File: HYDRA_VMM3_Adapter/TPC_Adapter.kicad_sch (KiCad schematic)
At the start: 1 part

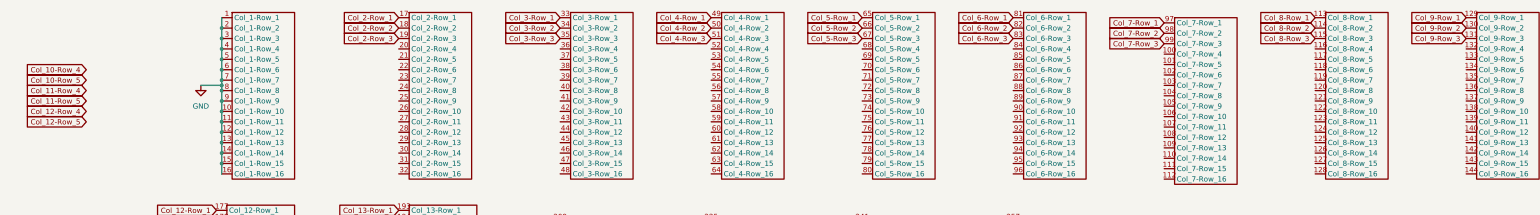
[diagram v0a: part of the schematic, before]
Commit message: .
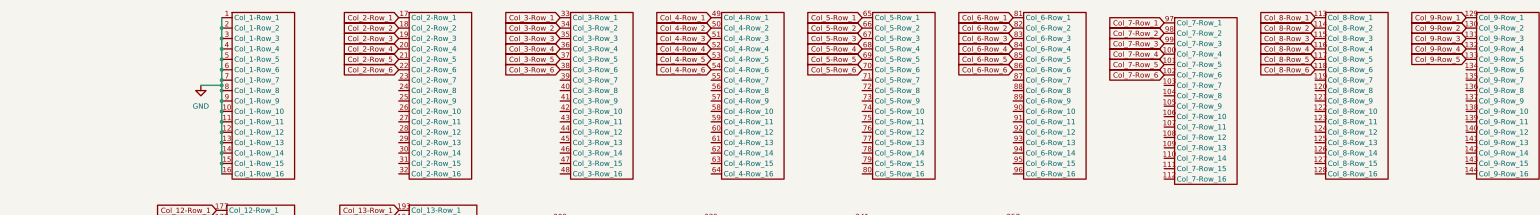
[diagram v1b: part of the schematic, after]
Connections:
- net Col_7-Row_4: now reaches U1.100 (Col_7-Row_4)
- net Col_7-Row_5: now reaches U1.101 (Col_7-Row_5)
- net Col_7-Row_6: now reaches U1.102 (Col_7-Row_6)
- net Col_8-Row_4: now reaches U1.116 (Col_8-Row_4)
- net Col_8-Row_5: now reaches U1.117 (Col_8-Row_5)
- net Col_8-Row_6: now reaches U1.118 (Col_8-Row_6)
- net Col_9-Row_4: now reaches U1.132 (Col_9-Row_4)
- net Col_9-Row_5: now reaches U1.133 (Col_9-Row_5)
- net Col_2-Row_4: now reaches U1.20 (Col_2-Row_4)
- net Col_2-Row_5: now reaches U1.21 (Col_2-Row_5)
- net Col_2-Row_6: now reaches U1.22 (Col_2-Row_6)
- net Col_3-Row_4: now reaches U1.36 (Col_3-Row_4)
- net Col_3-Row_5: now reaches U1.37 (Col_3-Row_5)
- net Col_3-Row_6: now reaches U1.38 (Col_3-Row_6)
- net Col_4-Row_4: now reaches U1.52 (Col_4-Row_4)
- net Col_4-Row_5: now reaches U1.53 (Col_4-Row_5)
- net Col_4-Row_6: now reaches U1.54 (Col_4-Row_6)
- net Col_5-Row_4: now reaches U1.68 (Col_5-Row_4)
- net Col_5-Row_5: now reaches U1.69 (Col_5-Row_5)
- net Col_5-Row_6: now reaches U1.70 (Col_5-Row_6)
- net Col_6-Row_4: now reaches U1.84 (Col_6-Row_4)
- net Col_6-Row_5: now reaches U1.85 (Col_6-Row_5)
- net Col_6-Row_6: now reaches U1.86 (Col_6-Row_6)

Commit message: .
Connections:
- net Col_23-Row_1: now reaches U1.353 (Col_23-Row_1)
- net Col_23-Row_2: now reaches U1.354 (Col_23-Row_2)
- net Col_23-Row_3: now reaches U1.355 (Col_23-Row_3)
- net Col_23-Row_4: now reaches U1.356 (Col_23-Row_4)
- net Col_23-Row_5: now reaches U1.357 (Col_23-Row_5)
- net Col_24-Row_1: now reaches U1.369 (Col_24-Row_1)
- net Col_24-Row_2: now reaches U1.370 (Col_24-Row_2)
- net Col_24-Row_3: now reaches U1.371 (Col_24-Row_3)
- net Col_24-Row_4: now reaches U1.372 (Col_24-Row_4)
- net Col_24-Row_5: now reaches U1.373 (Col_24-Row_5)
- net Col_25-Row_1: now reaches U1.385 (Col_25-Row_1)
- net Col_25-Row_2: now reaches U1.386 (Col_25-Row_2)
- net Col_25-Row_3: now reaches U1.387 (Col_25-Row_3)
- net Col_25-Row_4: now reaches U1.388 (Col_25-Row_4)
- net Col_25-Row_5: now reaches U1.389 (Col_25-Row_5)
- net Col_26-Row_1: now reaches U1.401 (Col_26-Row_1)
- net Col_26-Row_2: now reaches U1.402 (Col_26-Row_2)
- net Col_26-Row_3: now reaches U1.403 (Col_26-Row_3)
- net Col_26-Row_4: now reaches U1.404 (Col_26-Row_4)
- net Col_26-Row_5: now reaches U1.405 (Col_26-Row_5)
- net Col_27-Row_1: now reaches U1.417 (Col_27-Row_1)
- net Col_27-Row_2: now reaches U1.418 (Col_27-Row_2)
- net Col_27-Row_3: now reaches U1.419 (Col_27-Row_3)
- net Col_27-Row_4: now reaches U1.420 (Col_27-Row_4)
- net Col_27-Row_5: now reaches U1.421 (Col_27-Row_5)
- net Col_28-Row_1: now reaches U1.433 (Col_28-Row_1)
- net Col_28-Row_2: now reaches U1.434 (Col_28-Row_2)
- net Col_28-Row_3: now reaches U1.435 (Col_28-Row_3)
- net Col_28-Row_4: now reaches U1.436 (Col_28-Row_4)
- net Col_28-Row_5: now reaches U1.437 (Col_28-Row_5)
- net Col_29-Row_1: now reaches U1.449 (Col_29-Row_1)
- net Col_29-Row_2: now reaches U1.450 (Col_29-Row_2)
- net Col_29-Row_3: now reaches U1.451 (Col_29-Row_3)
- net Col_29-Row_4: now reaches U1.452 (Col_29-Row_4)
- net Col_29-Row_5: now reaches U1.453 (Col_29-Row_5)
- net Col_30-Row_1: now reaches U1.465 (Col_30-Row_1)
- net Col_30-Row_2: now reaches U1.466 (Col_30-Row_2)
- net Col_30-Row_3: now reaches U1.467 (Col_30-Row_3)
- net Col_30-Row_4: now reaches U1.468 (Col_30-Row_4)
- net Col_30-Row_5: now reaches U1.469 (Col_30-Row_5)
- net Col_31-Row_1: now reaches U1.481 (Col_31-Row_1)
- net Col_31-Row_2: now reaches U1.482 (Col_31-Row_2)
- net Col_31-Row_3: now reaches U1.483 (Col_31-Row_3)
- net Col_31-Row_4: now reaches U1.484 (Col_31-Row_4)
- net Col_31-Row_5: now reaches U1.485 (Col_31-Row_5)
- net Col_32-Row_1: now reaches U1.497 (Col_32-Row_1)
- net Col_32-Row_2: now reaches U1.498 (Col_32-Row_2)
- net Col_32-Row_3: now reaches U1.499 (Col_32-Row_3)
- net Col_32-Row_4: now reaches U1.500 (Col_32-Row_4)
- net Col_32-Row_5: now reaches U1.501 (Col_32-Row_5)
- net Col_33-Row_1: now reaches U1.513 (Col_33-Row_1)
- net Col_33-Row_2: now reaches U1.514 (Col_33-Row_2)
- net Col_33-Row_3: now reaches U1.515 (Col_33-Row_3)
- net Col_33-Row_4: now reaches U1.516 (Col_33-Row_4)
- net Col_33-Row_5: now reaches U1.517 (Col_33-Row_5)
- net Col_34-Row_1: now reaches U1.529 (Col_34-Row_1)
- net Col_34-Row_2: now reaches U1.530 (Col_34-Row_2)
- net Col_34-Row_3: now reaches U1.531 (Col_34-Row_3)
- net Col_34-Row_4: now reaches U1.532 (Col_34-Row_4)
- net Col_34-Row_5: now reaches U1.533 (Col_34-Row_5)
- net Col_35-Row_1: now reaches U1.545 (Col_35-Row_1)
- net Col_35-Row_2: now reaches U1.546 (Col_35-Row_2)
- net Col_35-Row_3: now reaches U1.547 (Col_35-Row_3)
- net Col_35-Row_4: now reaches U1.548 (Col_35-Row_4)
- net Col_35-Row_5: now reaches U1.549 (Col_35-Row_5)
- net Col_36-Row_1: now reaches U1.561 (Col_36-Row_1)
- net Col_36-Row_2: now reaches U1.562 (Col_36-Row_2)
- net Col_36-Row_3: now reaches U1.563 (Col_36-Row_3)
- net Col_36-Row_4: now reaches U1.564 (Col_36-Row_4)
- net Col_36-Row_5: now reaches U1.565 (Col_36-Row_5)
- net Col_37-Row_1: now reaches U1.577 (Col_37-Row_1)
- net Col_37-Row_2: now reaches U1.578 (Col_37-Row_2)
- net Col_37-Row_3: now reaches U1.579 (Col_37-Row_3)
- net Col_37-Row_4: now reaches U1.580 (Col_37-Row_4)
- net Col_37-Row_5: now reaches U1.581 (Col_37-Row_5)
- net Col_37-Row_6: now reaches U1.582 (Col_37-Row_6)
- net Col_38-Row_1: now reaches U1.593 (Col_38-Row_1)
- net Col_38-Row_2: now reaches U1.594 (Col_38-Row_2)
- net Col_38-Row_3: now reaches U1.595 (Col_38-Row_3)
- net Col_38-Row_4: now reaches U1.596 (Col_38-Row_4)
- net Col_38-Row_5: now reaches U1.597 (Col_38-Row_5)
- net Col_38-Row_6: now reaches U1.598 (Col_38-Row_6)
- net Col_39-Row_1: now reaches U1.609 (Col_39-Row_1)
- net Col_39-Row_2: now reaches U1.610 (Col_39-Row_2)
- net Col_39-Row_3: now reaches U1.611 (Col_39-Row_3)
- net Col_39-Row_4: now reaches U1.612 (Col_39-Row_4)
- net Col_39-Row_5: now reaches U1.613 (Col_39-Row_5)
- net Col_39-Row_6: now reaches U1.614 (Col_39-Row_6)
- net Col_40-Row_1: now reaches U1.625 (Col_40-Row_1)
- net Col_40-Row_2: now reaches U1.626 (Col_40-Row_2)
- net Col_40-Row_3: now reaches U1.627 (Col_40-Row_3)
- net Col_40-Row_4: now reaches U1.628 (Col_40-Row_4)
- net Col_40-Row_5: now reaches U1.629 (Col_40-Row_5)
- net Col_40-Row_6: now reaches U1.630 (Col_40-Row_6)
- net Col_41-Row_1: now reaches U1.641 (Col_41-Row_1)
- net Col_41-Row_2: now reaches U1.642 (Col_41-Row_2)
- net Col_41-Row_3: now reaches U1.643 (Col_41-Row_3)
- net Col_41-Row_4: now reaches U1.644 (Col_41-Row_4)
- net Col_41-Row_5: now reaches U1.645 (Col_41-Row_5)
- net Col_41-Row_6: now reaches U1.646 (Col_41-Row_6)
- net Col_42-Row_1: now reaches U1.657 (Col_42-Row_1)
- net Col_42-Row_2: now reaches U1.658 (Col_42-Row_2)
- net Col_42-Row_3: now reaches U1.659 (Col_42-Row_3)
- net Col_42-Row_4: now reaches U1.660 (Col_42-Row_4)
- net Col_42-Row_5: now reaches U1.661 (Col_42-Row_5)
- net Col_42-Row_6: now reaches U1.662 (Col_42-Row_6)
- net Col_43-Row_1: now reaches U1.673 (Col_43-Row_1)
- net Col_43-Row_2: now reaches U1.674 (Col_43-Row_2)
- net Col_43-Row_3: now reaches U1.675 (Col_43-Row_3)
- net Col_43-Row_4: now reaches U1.676 (Col_43-Row_4)
- net Col_43-Row_5: now reaches U1.677 (Col_43-Row_5)
- net Col_43-Row_6: now reaches U1.678 (Col_43-Row_6)

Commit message: .
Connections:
- net Col_7-Row_12: now reaches U1.108 (Col_7-Row_12)
- net Col_7-Row_13: now reaches U1.109 (Col_7-Row_13)
- net Col_7-Row_14: now reaches U1.110 (Col_7-Row_14)
- net Col_7-Row_15: now reaches U1.111 (Col_7-Row_15)
- net Col_7-Row_16: now reaches U1.112 (Col_7-Row_16)
- net Col_8-Row_12: now reaches U1.124 (Col_8-Row_12)
- net Col_8-Row_13: now reaches U1.125 (Col_8-Row_13)
- net Col_8-Row_14: now reaches U1.126 (Col_8-Row_14)
- net Col_8-Row_15: now reaches U1.127 (Col_8-Row_15)
- net Col_8-Row_16: now reaches U1.128 (Col_8-Row_16)
- net Col_9-Row_12: now reaches U1.140 (Col_9-Row_12)
- net Col_9-Row_13: now reaches U1.141 (Col_9-Row_13)
- net Col_9-Row_14: now reaches U1.142 (Col_9-Row_14)
- net Col_9-Row_15: now reaches U1.143 (Col_9-Row_15)
- net Col_9-Row_16: now reaches U1.144 (Col_9-Row_16)
- net Col_10-Row_12: now reaches U1.156 (Col_10-Row_12)
- net Col_10-Row_13: now reaches U1.157 (Col_10-Row_13)
- net Col_10-Row_14: now reaches U1.158 (Col_10-Row_14)
- net Col_10-Row_15: now reaches U1.159 (Col_10-Row_15)
- net Col_10-Row_16: now reaches U1.160 (Col_10-Row_16)
- net Col_11-Row_12: now reaches U1.172 (Col_11-Row_12)
- net Col_11-Row_13: now reaches U1.173 (Col_11-Row_13)
- net Col_11-Row_14: now reaches U1.174 (Col_11-Row_14)
- net Col_11-Row_15: now reaches U1.175 (Col_11-Row_15)
- net Col_11-Row_16: now reaches U1.176 (Col_11-Row_16)
- net Col_12-Row_12: now reaches U1.188 (Col_12-Row_12)
- net Col_12-Row_13: now reaches U1.189 (Col_12-Row_13)
- net Col_12-Row_14: now reaches U1.190 (Col_12-Row_14)
- net Col_12-Row_15: now reaches U1.191 (Col_12-Row_15)
- net Col_12-Row_16: now reaches U1.192 (Col_12-Row_16)
- net Col_13-Row_12: now reaches U1.204 (Col_13-Row_12)
- net Col_13-Row_13: now reaches U1.205 (Col_13-Row_13)
- net Col_13-Row_14: now reaches U1.206 (Col_13-Row_14)
- net Col_13-Row_15: now reaches U1.207 (Col_13-Row_15)
- net Col_13-Row_16: now reaches U1.208 (Col_13-Row_16)
- net Col_14-Row_12: now reaches U1.220 (Col_14-Row_12)
- net Col_14-Row_13: now reaches U1.221 (Col_14-Row_13)
- net Col_14-Row_14: now reaches U1.222 (Col_14-Row_14)
- net Col_14-Row_15: now reaches U1.223 (Col_14-Row_15)
- net Col_14-Row_16: now reaches U1.224 (Col_14-Row_16)
- net Col_15-Row_12: now reaches U1.236 (Col_15-Row_12)
- net Col_15-Row_13: now reaches U1.237 (Col_15-Row_13)
- net Col_15-Row_14: now reaches U1.238 (Col_15-Row_14)
- net Col_15-Row_15: now reaches U1.239 (Col_15-Row_15)
- net Col_15-Row_16: now reaches U1.240 (Col_15-Row_16)
- net Col_16-Row_11: now reaches U1.251 (Col_16-Row_11)
- net Col_16-Row_12: now reaches U1.252 (Col_16-Row_12)
- net Col_16-Row_13: now reaches U1.253 (Col_16-Row_13)
- net Col_16-Row_14: now reaches U1.254 (Col_16-Row_14)
- net Col_16-Row_15: now reaches U1.255 (Col_16-Row_15)
- net Col_16-Row_16: now reaches U1.256 (Col_16-Row_16)
- net Col_17-Row_11: now reaches U1.267 (Col_17-Row_11)
- net Col_17-Row_12: now reaches U1.268 (Col_17-Row_12)
- net Col_17-Row_13: now reaches U1.269 (Col_17-Row_13)
- net Col_17-Row_14: now reaches U1.270 (Col_17-Row_14)
- net Col_17-Row_15: now reaches U1.271 (Col_17-Row_15)
- net Col_17-Row_16: now reaches U1.272 (Col_17-Row_16)
- net Col_2-Row_12: now reaches U1.28 (Col_2-Row_12)
- net Col_18-Row_11: now reaches U1.283 (Col_18-Row_11)
- net Col_18-Row_12: now reaches U1.284 (Col_18-Row_12)
- net Col_18-Row_13: now reaches U1.285 (Col_18-Row_13)
- net Col_18-Row_14: now reaches U1.286 (Col_18-Row_14)
- net Col_18-Row_15: now reaches U1.287 (Col_18-Row_15)
- net Col_18-Row_16: now reaches U1.288 (Col_18-Row_16)
- net Col_2-Row_13: now reaches U1.29 (Col_2-Row_13)
- net Col_19-Row_11: now reaches U1.299 (Col_19-Row_11)
- net Col_2-Row_14: now reaches U1.30 (Col_2-Row_14)
- net Col_19-Row_12: now reaches U1.300 (Col_19-Row_12)
- net Col_19-Row_13: now reaches U1.301 (Col_19-Row_13)
- net Col_19-Row_14: now reaches U1.302 (Col_19-Row_14)
- net Col_19-Row_15: now reaches U1.303 (Col_19-Row_15)
- net Col_19-Row_16: now reaches U1.304 (Col_19-Row_16)
- net Col_2-Row_15: now reaches U1.31 (Col_2-Row_15)
- net Col_20-Row_11: now reaches U1.315 (Col_20-Row_11)
- net Col_20-Row_12: now reaches U1.316 (Col_20-Row_12)
- net Col_20-Row_13: now reaches U1.317 (Col_20-Row_13)
- net Col_20-Row_14: now reaches U1.318 (Col_20-Row_14)
- net Col_20-Row_15: now reaches U1.319 (Col_20-Row_15)
- net Col_2-Row_16: now reaches U1.32 (Col_2-Row_16)
- net Col_20-Row_16: now reaches U1.320 (Col_20-Row_16)
- net Col_21-Row_11: now reaches U1.331 (Col_21-Row_11)
- net Col_21-Row_12: now reaches U1.332 (Col_21-Row_12)
- net Col_21-Row_13: now reaches U1.333 (Col_21-Row_13)
- net Col_21-Row_14: now reaches U1.334 (Col_21-Row_14)
- net Col_21-Row_15: now reaches U1.335 (Col_21-Row_15)
- net Col_21-Row_16: now reaches U1.336 (Col_21-Row_16)
- net Col_22-Row_11: now reaches U1.347 (Col_22-Row_11)
- net Col_22-Row_12: now reaches U1.348 (Col_22-Row_12)
- net Col_22-Row_13: now reaches U1.349 (Col_22-Row_13)
- net Col_22-Row_14: now reaches U1.350 (Col_22-Row_14)
- net Col_22-Row_15: now reaches U1.351 (Col_22-Row_15)
- net Col_22-Row_16: now reaches U1.352 (Col_22-Row_16)
- net Col_3-Row_12: now reaches U1.44 (Col_3-Row_12)
- net Col_3-Row_13: now reaches U1.45 (Col_3-Row_13)
- net Col_3-Row_14: now reaches U1.46 (Col_3-Row_14)
- net Col_3-Row_15: now reaches U1.47 (Col_3-Row_15)
- net Col_3-Row_16: now reaches U1.48 (Col_3-Row_16)
- net Col_4-Row_12: now reaches U1.60 (Col_4-Row_12)
- net Col_4-Row_13: now reaches U1.61 (Col_4-Row_13)
- net Col_4-Row_14: now reaches U1.62 (Col_4-Row_14)
- net Col_4-Row_15: now reaches U1.63 (Col_4-Row_15)
- net Col_4-Row_16: now reaches U1.64 (Col_4-Row_16)
- net Col_5-Row_12: now reaches U1.76 (Col_5-Row_12)
- net Col_5-Row_13: now reaches U1.77 (Col_5-Row_13)
- net Col_5-Row_14: now reaches U1.78 (Col_5-Row_14)
- net Col_5-Row_15: now reaches U1.79 (Col_5-Row_15)
- net Col_5-Row_16: now reaches U1.80 (Col_5-Row_16)
- net Col_6-Row_12: now reaches U1.92 (Col_6-Row_12)
- net Col_6-Row_13: now reaches U1.93 (Col_6-Row_13)
- net Col_6-Row_14: now reaches U1.94 (Col_6-Row_14)
- net Col_6-Row_15: now reaches U1.95 (Col_6-Row_15)
- net Col_6-Row_16: now reaches U1.96 (Col_6-Row_16)

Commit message: .
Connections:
- net Col_23-Row_11: now reaches U1.363 (Col_23-Row_11)
- net Col_23-Row_12: now reaches U1.364 (Col_23-Row_12)
- net Col_23-Row_13: now reaches U1.365 (Col_23-Row_13)
- net Col_23-Row_14: now reaches U1.366 (Col_23-Row_14)
- net Col_23-Row_15: now reaches U1.367 (Col_23-Row_15)
- net Col_23-Row_16: now reaches U1.368 (Col_23-Row_16)
- net Col_24-Row_11: now reaches U1.379 (Col_24-Row_11)
- net Col_24-Row_12: now reaches U1.380 (Col_24-Row_12)
- net Col_24-Row_13: now reaches U1.381 (Col_24-Row_13)
- net Col_24-Row_14: now reaches U1.382 (Col_24-Row_14)
- net Col_24-Row_15: now reaches U1.383 (Col_24-Row_15)
- net Col_24-Row_16: now reaches U1.384 (Col_24-Row_16)
- net Col_25-Row_11: now reaches U1.395 (Col_25-Row_11)
- net Col_25-Row_12: now reaches U1.396 (Col_25-Row_12)
- net Col_25-Row_13: now reaches U1.397 (Col_25-Row_13)
- net Col_25-Row_14: now reaches U1.398 (Col_25-Row_14)
- net Col_25-Row_15: now reaches U1.399 (Col_25-Row_15)
- net Col_25-Row_16: now reaches U1.400 (Col_25-Row_16)
- net Col_26-Row_11: now reaches U1.411 (Col_26-Row_11)
- net Col_26-Row_12: now reaches U1.412 (Col_26-Row_12)
- net Col_26-Row_13: now reaches U1.413 (Col_26-Row_13)
- net Col_26-Row_14: now reaches U1.414 (Col_26-Row_14)
- net Col_26-Row_15: now reaches U1.415 (Col_26-Row_15)
- net Col_26-Row_16: now reaches U1.416 (Col_26-Row_16)
- net Col_27-Row_11: now reaches U1.427 (Col_27-Row_11)
- net Col_27-Row_12: now reaches U1.428 (Col_27-Row_12)
- net Col_27-Row_13: now reaches U1.429 (Col_27-Row_13)
- net Col_27-Row_14: now reaches U1.430 (Col_27-Row_14)
- net Col_27-Row_15: now reaches U1.431 (Col_27-Row_15)
- net Col_27-Row_16: now reaches U1.432 (Col_27-Row_16)
- net Col_28-Row_11: now reaches U1.443 (Col_28-Row_11)
- net Col_28-Row_12: now reaches U1.444 (Col_28-Row_12)
- net Col_28-Row_13: now reaches U1.445 (Col_28-Row_13)
- net Col_28-Row_14: now reaches U1.446 (Col_28-Row_14)
- net Col_28-Row_15: now reaches U1.447 (Col_28-Row_15)
- net Col_28-Row_16: now reaches U1.448 (Col_28-Row_16)
- net Col_29-Row_11: now reaches U1.459 (Col_29-Row_11)
- net Col_29-Row_12: now reaches U1.460 (Col_29-Row_12)
- net Col_29-Row_13: now reaches U1.461 (Col_29-Row_13)
- net Col_29-Row_14: now reaches U1.462 (Col_29-Row_14)
- net Col_29-Row_15: now reaches U1.463 (Col_29-Row_15)
- net Col_29-Row_16: now reaches U1.464 (Col_29-Row_16)
- net Col_30-Row_12: now reaches U1.476 (Col_30-Row_12)
- net Col_30-Row_13: now reaches U1.477 (Col_30-Row_13)
- net Col_30-Row_14: now reaches U1.478 (Col_30-Row_14)
- net Col_30-Row_15: now reaches U1.479 (Col_30-Row_15)
- net Col_30-Row_16: now reaches U1.480 (Col_30-Row_16)
- net Col_31-Row_12: now reaches U1.492 (Col_31-Row_12)
- net Col_31-Row_13: now reaches U1.493 (Col_31-Row_13)
- net Col_31-Row_14: now reaches U1.494 (Col_31-Row_14)
- net Col_31-Row_15: now reaches U1.495 (Col_31-Row_15)
- net Col_31-Row_16: now reaches U1.496 (Col_31-Row_16)
- net Col_32-Row_12: now reaches U1.508 (Col_32-Row_12)
- net Col_32-Row_13: now reaches U1.509 (Col_32-Row_13)
- net Col_32-Row_14: now reaches U1.510 (Col_32-Row_14)
- net Col_32-Row_15: now reaches U1.511 (Col_32-Row_15)
- net Col_32-Row_16: now reaches U1.512 (Col_32-Row_16)
- net Col_33-Row_12: now reaches U1.524 (Col_33-Row_12)
- net Col_33-Row_13: now reaches U1.525 (Col_33-Row_13)
- net Col_33-Row_14: now reaches U1.526 (Col_33-Row_14)
- net Col_33-Row_15: now reaches U1.527 (Col_33-Row_15)
- net Col_33-Row_16: now reaches U1.528 (Col_33-Row_16)
- net Col_34-Row_12: now reaches U1.540 (Col_34-Row_12)
- net Col_34-Row_13: now reaches U1.541 (Col_34-Row_13)
- net Col_34-Row_14: now reaches U1.542 (Col_34-Row_14)
- net Col_34-Row_15: now reaches U1.543 (Col_34-Row_15)
- net Col_34-Row_16: now reaches U1.544 (Col_34-Row_16)
- net Col_35-Row_12: now reaches U1.556 (Col_35-Row_12)
- net Col_35-Row_13: now reaches U1.557 (Col_35-Row_13)
- net Col_35-Row_14: now reaches U1.558 (Col_35-Row_14)
- net Col_35-Row_15: now reaches U1.559 (Col_35-Row_15)
- net Col_35-Row_16: now reaches U1.560 (Col_35-Row_16)
- net Col_36-Row_12: now reaches U1.572 (Col_36-Row_12)
- net Col_36-Row_13: now reaches U1.573 (Col_36-Row_13)
- net Col_36-Row_14: now reaches U1.574 (Col_36-Row_14)
- net Col_36-Row_15: now reaches U1.575 (Col_36-Row_15)
- net Col_36-Row_16: now reaches U1.576 (Col_36-Row_16)
- net Col_37-Row_12: now reaches U1.588 (Col_37-Row_12)
- net Col_37-Row_13: now reaches U1.589 (Col_37-Row_13)
- net Col_37-Row_14: now reaches U1.590 (Col_37-Row_14)
- net Col_37-Row_15: now reaches U1.591 (Col_37-Row_15)
- net Col_37-Row_16: now reaches U1.592 (Col_37-Row_16)
- net Col_38-Row_12: now reaches U1.604 (Col_38-Row_12)
- net Col_38-Row_13: now reaches U1.605 (Col_38-Row_13)
- net Col_38-Row_14: now reaches U1.606 (Col_38-Row_14)
- net Col_38-Row_15: now reaches U1.607 (Col_38-Row_15)
- net Col_38-Row_16: now reaches U1.608 (Col_38-Row_16)
- net Col_39-Row_12: now reaches U1.620 (Col_39-Row_12)
- net Col_39-Row_13: now reaches U1.621 (Col_39-Row_13)
- net Col_39-Row_14: now reaches U1.622 (Col_39-Row_14)
- net Col_39-Row_15: now reaches U1.623 (Col_39-Row_15)
- net Col_39-Row_16: now reaches U1.624 (Col_39-Row_16)
- net Col_40-Row_12: now reaches U1.636 (Col_40-Row_12)
- net Col_40-Row_13: now reaches U1.637 (Col_40-Row_13)
- net Col_40-Row_14: now reaches U1.638 (Col_40-Row_14)
- net Col_40-Row_15: now reaches U1.639 (Col_40-Row_15)
- net Col_40-Row_16: now reaches U1.640 (Col_40-Row_16)
- net Col_41-Row_12: now reaches U1.652 (Col_41-Row_12)
- net Col_41-Row_13: now reaches U1.653 (Col_41-Row_13)
- net Col_41-Row_14: now reaches U1.654 (Col_41-Row_14)
- net Col_41-Row_15: now reaches U1.655 (Col_41-Row_15)
- net Col_41-Row_16: now reaches U1.656 (Col_41-Row_16)
- net Col_42-Row_12: now reaches U1.668 (Col_42-Row_12)
- net Col_42-Row_13: now reaches U1.669 (Col_42-Row_13)
- net Col_42-Row_14: now reaches U1.670 (Col_42-Row_14)
- net Col_42-Row_15: now reaches U1.671 (Col_42-Row_15)
- net Col_42-Row_16: now reaches U1.672 (Col_42-Row_16)
- net Col_43-Row_12: now reaches U1.684 (Col_43-Row_12)
- net Col_43-Row_13: now reaches U1.685 (Col_43-Row_13)
- net Col_43-Row_14: now reaches U1.686 (Col_43-Row_14)
- net Col_43-Row_15: now reaches U1.687 (Col_43-Row_15)
- net Col_43-Row_16: now reaches U1.688 (Col_43-Row_16)
